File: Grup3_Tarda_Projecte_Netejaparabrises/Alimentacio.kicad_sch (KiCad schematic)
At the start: 10 parts, among them IC1 L78S05CV, J1 Screw_Terminal_01x02

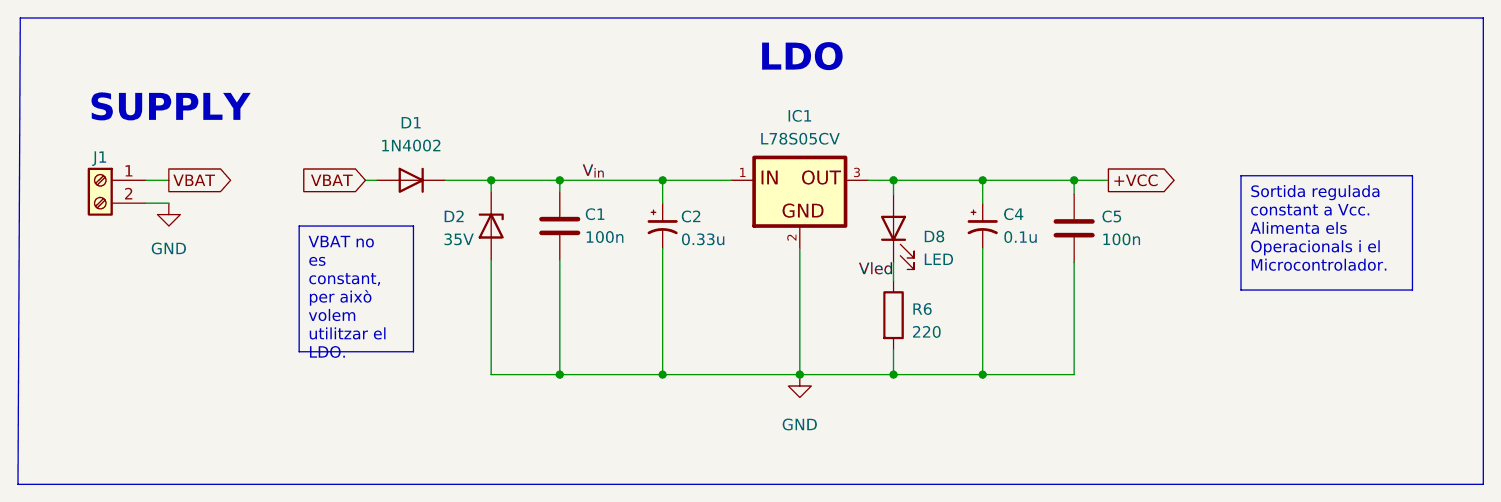
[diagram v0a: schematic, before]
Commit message: canvis reles 07-04-2023
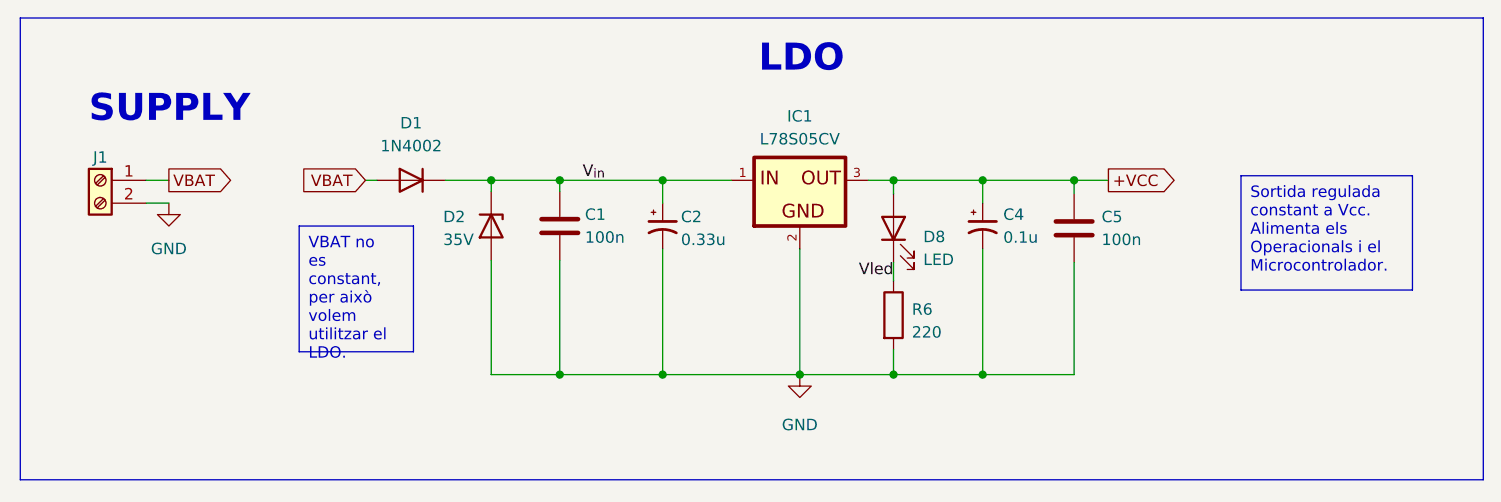
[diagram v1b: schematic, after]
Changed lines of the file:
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@@
     (stroke (width 0) (type default))
   )
-  (polyline (pts (xy 60.96 44.958) (xy 60.706 96.774))
+  (polyline (pts (xy 60.96 44.958) (xy 60.96 96.266))
     (stroke (width 0) (type default))
   )
@@
     (stroke (width 0) (type default))
   )
-  (polyline (pts (xy 223.52 96.774) (xy 60.706 96.774))
+  (polyline (pts (xy 223.52 96.266) (xy 60.96 96.266))
     (stroke (width 0) (type default))
   )
@@
     (stroke (width 0) (type default))
   )
-  (polyline (pts (xy 223.52 44.958) (xy 223.52 96.774))
+  (polyline (pts (xy 223.52 44.958) (xy 223.52 96.266))
     (stroke (width 0) (type default))
   )
